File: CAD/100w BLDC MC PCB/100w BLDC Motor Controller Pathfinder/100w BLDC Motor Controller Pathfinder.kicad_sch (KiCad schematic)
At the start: 37 parts, among them J1 USB_C_Receptacle_USB2.0, SW1 PTS815 SJM 250 SMTR LFS, U1 RP2040, U2 W25Q128JVS, U3 USBLC6-2SC6, U4 LMR36506MSC3RPERQ1, Y1 ABLS-12.000MHZ-B4-T

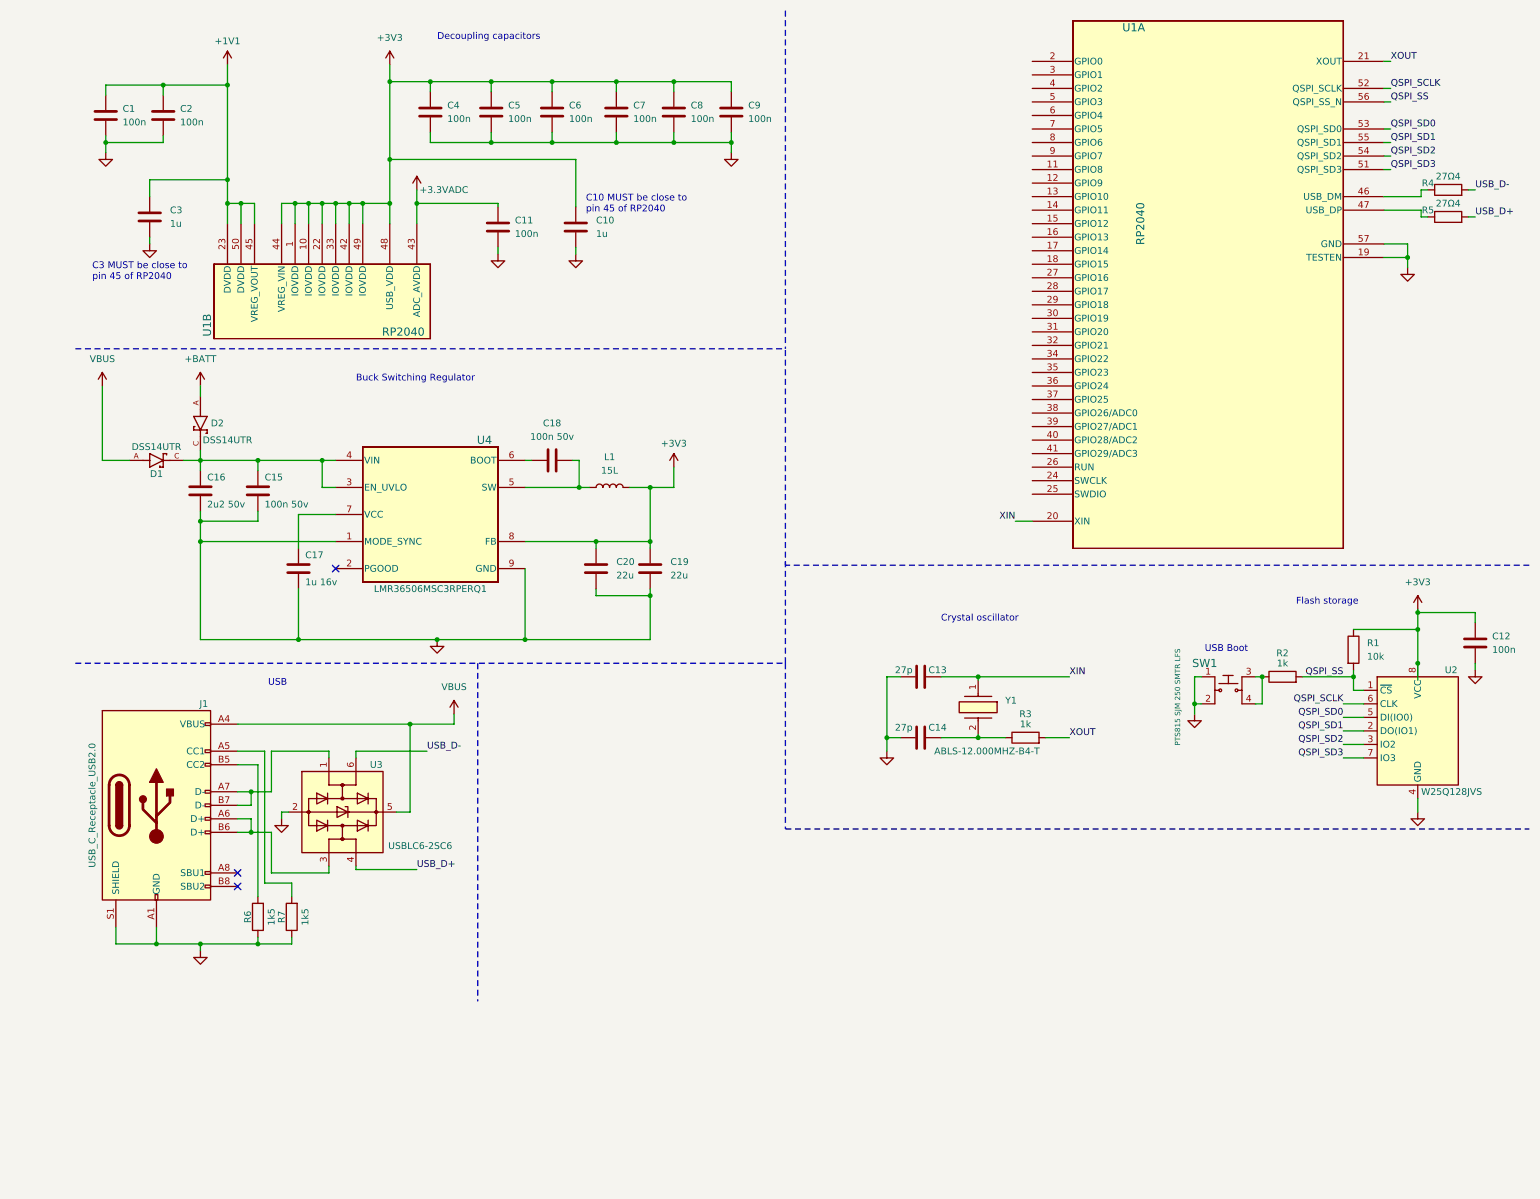
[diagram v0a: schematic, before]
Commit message: organización
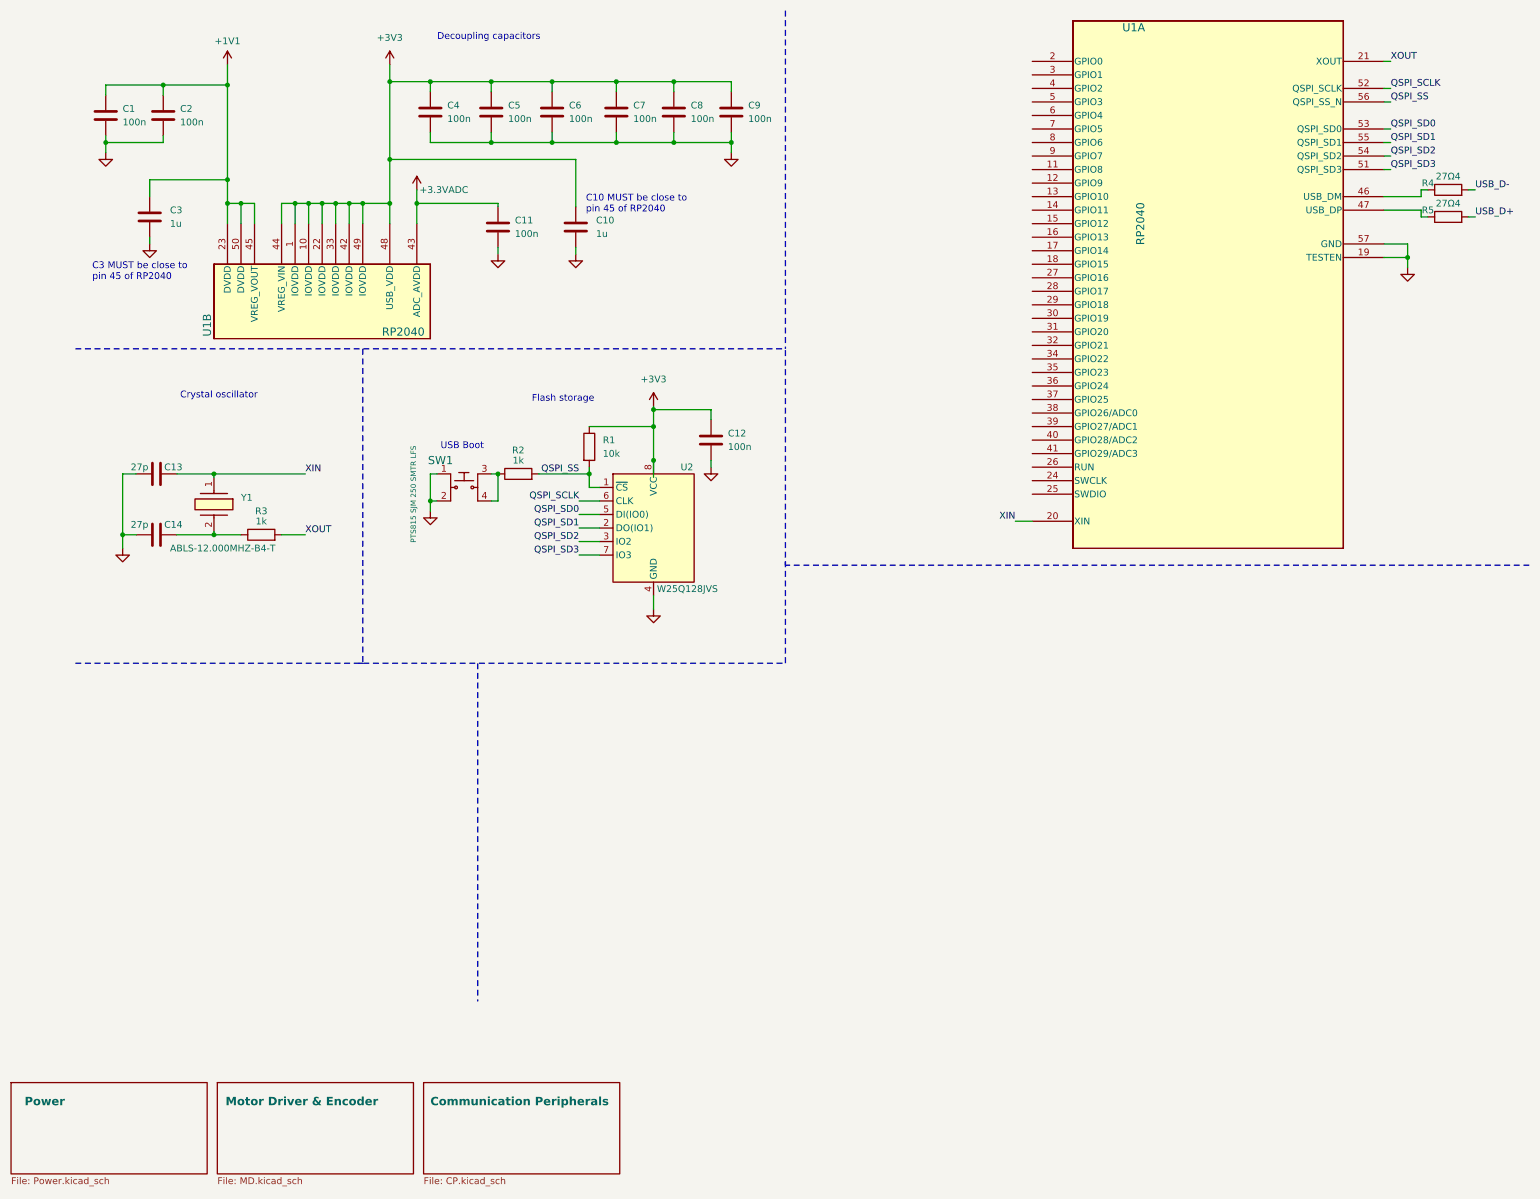
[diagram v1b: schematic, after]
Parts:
- removed C15, C18: 100n 50v, symbol Device:C
- removed C16: 2u2 50v, symbol Device:C
- removed C17: 1u 16v, symbol Device:C
- removed C19, C20: 22u, symbol Device:C
- removed D1, D2: DSS14UTR, DSS14UTR:SODFL3618X110N, symbol DSS14UTR:DSS14UTR
- removed J1: USB_C_Receptacle_USB2.0, symbol Connector:USB_C_Receptacle_USB2.0
- removed L1: 15L, symbol Device:L
- removed R6, R7: 1k5, symbol Device:R
- removed U3: USBLC6-2SC6, Package_TO_SOT_SMD:SOT-23-6, symbol Power_Protection:USBLC6-2SC6
- removed U4: LMR36506MSC3RPERQ1, RPE0009A, symbol 2024-01-23_05-03-01:LMR36506MSC3RPERQ1
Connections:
- no-connect marks 3 -> 0
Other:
- added sheet Communication Peripherals (CP.kicad_sch)
- added sheet Motor Driver & Encoder (MD.kicad_sch)
- added sheet Power (Power.kicad_sch)
- note removed: "Buck Switching Regulator"
- note removed: "USB"
- moved on the sheet: C12, C13, C14, R1, R2, R3, SW1, U2, Y1
